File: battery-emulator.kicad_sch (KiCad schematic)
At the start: 11 parts, among them U1 INA199A1DCKR

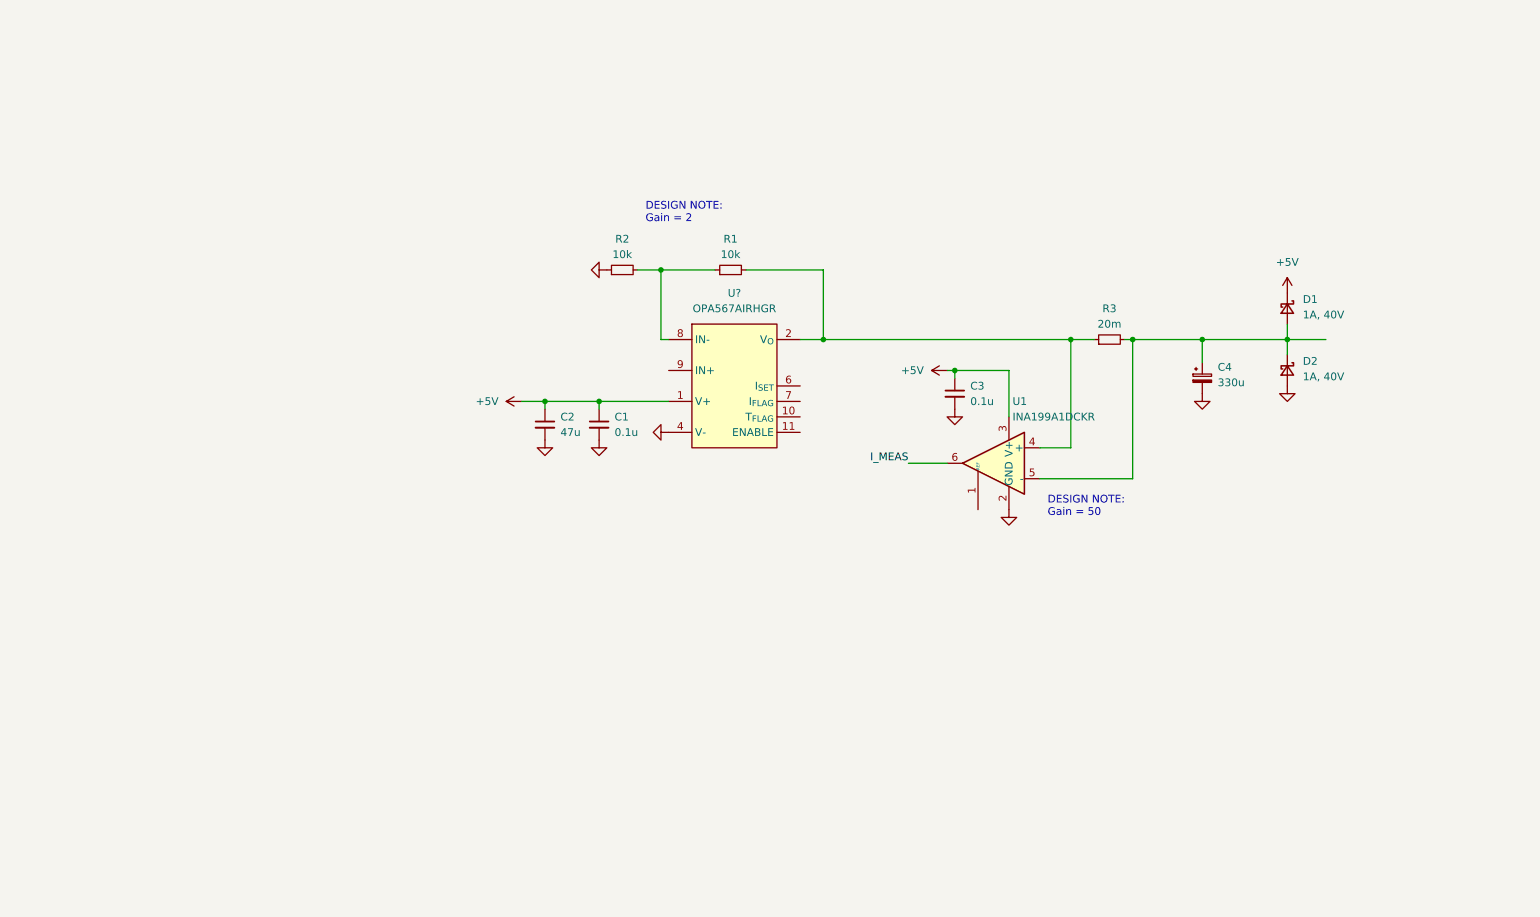
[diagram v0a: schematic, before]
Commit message: Some design
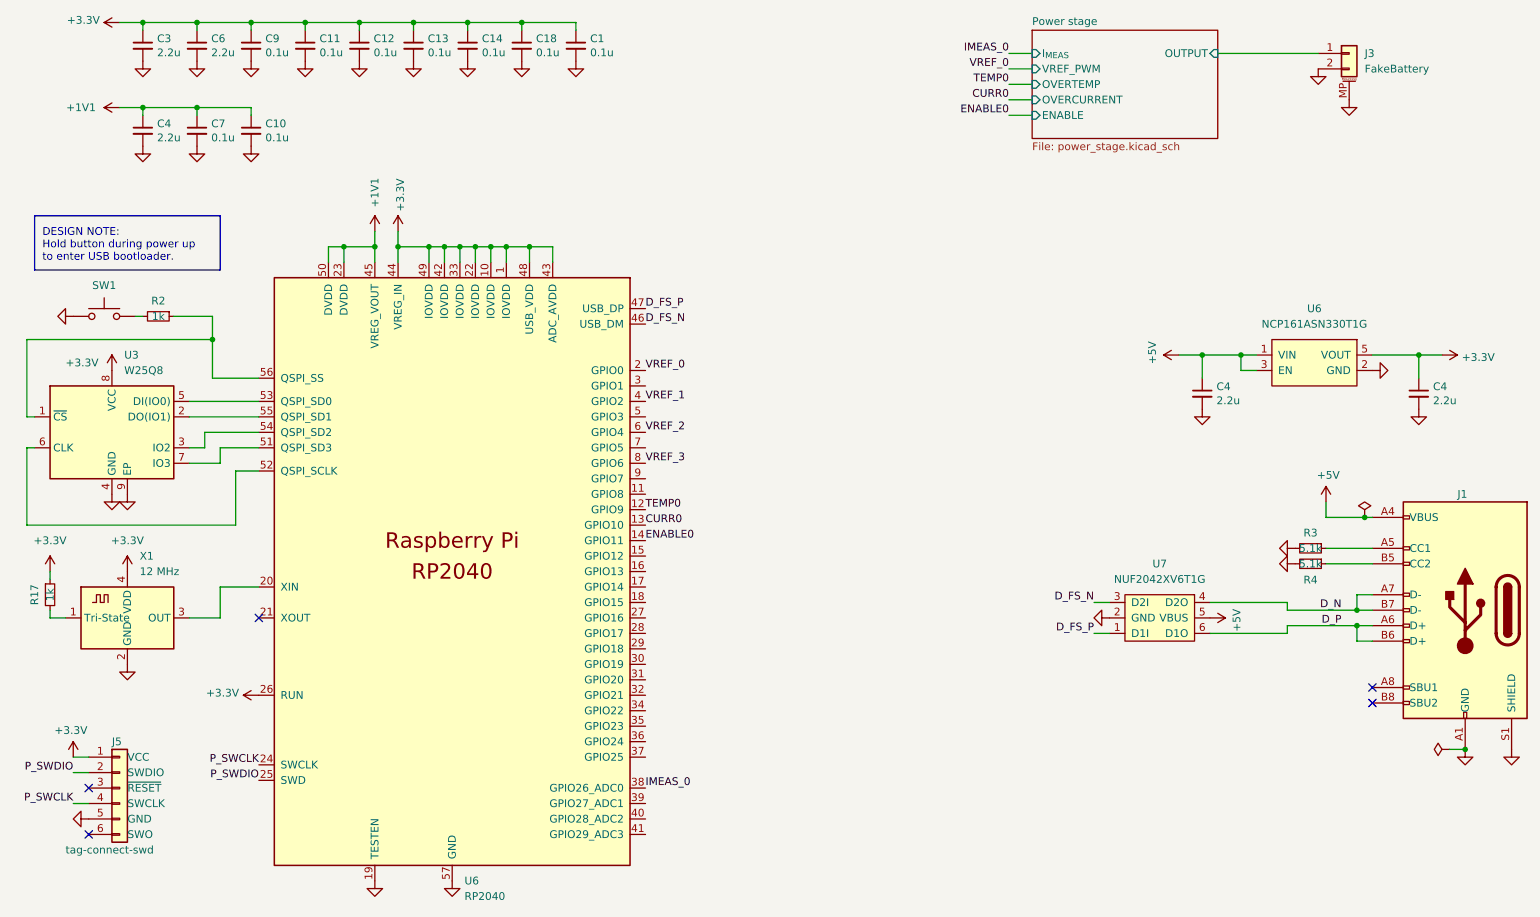
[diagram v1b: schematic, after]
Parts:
- removed C2: 47u, passive:C_1206, symbol Device:C_Small
- removed C4: 330u, Capacitor_SMD:C_Elec_8x10.2, symbol Device:C_Polarized_Small
- removed D1, D2: 1A, 40V, Diode_SMD:D_SOD-323, symbol Device:D_Schottky_Small
- removed R1: 10k, symbol Device:R_Small
- removed U1: INA199A1DCKR, Package_TO_SOT_SMD:SOT-363_SC-70-6, symbol Amplifier_Current:INA199xxDCK
- removed U?: OPA567AIRHGR, qfn:PVQFN-N12-1EP_5.0x5.0mm_P1.0mm_EP3.12x3.12mm, symbol opamp:OPA567
- added C10, C11, C12, C13, C14, C18, C7, C9: 0.1u, passive:C_0402, symbol Device:C_Small
- added C4 (x3), C6: 2.2u, passive:C_0402, symbol Device:C_Small
- added J1: USB_C_Receptacle_USB2.0, connectors:USB_C_Receptacle_USB4105, symbol Connector:USB_C_Receptacle_USB2.0
- added J3: FakeBattery, Connector_JST:JST_PH_S2B-PH-SM4-TB_1x02-1MP_P2.00mm_Horizontal, symbol Connector_Generic_MountingPin:Conn_01x02_MountingPin
- added J5: tag-connect-swd, Connector:Tag-Connect_TC2030-IDC-NL_2x03_P1.27mm_Vertical, symbol connectors:tag-connect-swd
- added R17: 1k, passive:R_0402, symbol Device:R_Small
- added R4: 5.1k, passive:R_0402, symbol Device:R_Small
- added SW1: SW_Push, Button_Switch_SMD:SW_SPST_EVQP2, symbol Switch:SW_Push
- added U3: W25Q8, son:USON-8-3x2mm-EP, symbol Memory_Flash:W25Q32JVZP
- added U6: RP2040, qfn:RP2040-QFN-56, symbol rp2040:RP2040
- added U6: NCP161ASN330T1G, sot:SOT-23-5, symbol ldo:NCP161ASN300T1G
- added U7: NUF2042XV6T1G, sot:SOT-563, symbol interface_esd:NUF2042XV6T1G
- added X1: 12 MHz, crystals:Crystal_SMD_2520-4Pin_2.5x2.0mm, symbol Oscillator:ASCO
- C1: LCSC (none) -> C56392; Tolerance (none) -> 25V, X7R
- C3: value 0.1u -> 2.2u; LCSC (none) -> C77002; Tolerance (none) -> 10V, X5R
- R2: value 10k -> 1k; footprint (none) -> passive:R_0402; LCSC (none) -> C106235; Tolerance (none) -> 1%
- R3: value 20m -> 5.1k; footprint (none) -> passive:R_0402; LCSC (none) -> C105872; Tolerance (none) -> 1%
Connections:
- net +5V: now also C4.1, J1.A4 (VBUS), J1.A9 (VBUS), J1.B4 (VBUS), J1.B9 (VBUS), U6.1 (VIN), U6.3 (EN), U7.5 (VBUS); no longer C1.1, C3.1
- net GND: now also R3.2, C10.2, C11.2, C12.2, C13.2, C14.2, C18.2, C4.2, C4.2, C4.2, C6.2, C7.2, C9.2, J1.A1 (GND), J1.A12 (GND), J1.B1 (GND), J1.B12 (GND), J1.S1 (SHIELD), J3.2 (Pin_2), J3.MP (MountPin), J5.5 (GND), R4.2, SW1.1, U3.4 (GND), U3.9 (EP), U6.19 (TESTEN), U6.2 (GND), U6.57 (GND), U7.2 (GND), X1.2 (GND); no longer R2.1
- net at R3.1: now also J1.A5 (CC1)
- net at R2.2: now also SW1.2
- new net: J1.B5 (CC2), R4.1
- new net: R17.2, X1.1 (Tri-State)
- new net: R2.1, U3.1 (~{CS}), U6.56 (QSPI_SS)
- new net: U6.20 (XIN), X1.3 (OUT)
- new net: U3.7 (IO3), U6.51 (QSPI_SD3)
- new net: U3.6 (CLK), U6.52 (QSPI_SCLK)
- new net: U3.5 (DI(IO0)), U6.53 (QSPI_SD0)
- new net: U3.3 (IO2), U6.54 (QSPI_SD2)
- new net: U3.2 (DO(IO1)), U6.55 (QSPI_SD1)
- new net +1V1: C10.1, C4.1, C7.1, U6.23 (DVDD), U6.45 (VREG_VOUT), U6.50 (DVDD)
- new net +3.3V: C1.1, C11.1, C12.1, C13.1, C14.1, C18.1, C3.1, C4.1, C6.1, C9.1, J5.1 (VCC), R17.1, U3.8 (VCC), U6.1 (IOVDD), U6.10 (IOVDD), U6.22 (IOVDD), U6.26 (RUN), U6.33 (IOVDD), U6.42 (IOVDD), U6.43 (ADC_AVDD), U6.44 (VREG_IN), U6.48 (USB_VDD), U6.49 (IOVDD), U6.5 (VOUT), X1.4 (VDD)
- new net CURR0: U6.13 (GPIO10)
- new net D_FS_N: U6.46 (USB_DM), U7.3 (D2I)
- new net D_FS_P: U6.47 (USB_DP), U7.1 (D1I)
- new net D_N: J1.A7 (D-), J1.B7 (D-), U7.4 (D2O)
- new net D_P: J1.A6 (D+), J1.B6 (D+), U7.6 (D1O)
- new net ENABLE0: U6.14 (GPIO11)
- new net IMEAS_0: U6.38 (GPIO26_ADC0)
- new net P_SWCLK: J5.4 (SWCLK), U6.24 (SWCLK)
- new net P_SWDIO: J5.2 (SWDIO), U6.25 (SWD)
- new net Power stage/OUTPUT: J3.1 (Pin_1)
- new net TEMP0: U6.12 (GPIO9)
- new net VREF_0: U6.2 (GPIO0)
- new net VREF_1: U6.4 (GPIO2)
- new net VREF_2: U6.6 (GPIO4)
- new net VREF_3: U6.8 (GPIO6)
- no-connect marks 0 -> 5
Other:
- added sheet Power stage (power_stage.kicad_sch)
- note added: "DESIGN NOTE: Hold button during power up to enter USB bootloader."
- note removed: "DESIGN NOTE: Gain = 2"
- note removed: "DESIGN NOTE: Gain = 50"
